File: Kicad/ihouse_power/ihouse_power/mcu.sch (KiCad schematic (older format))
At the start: 108 parts, among them J13 RJ33_Shielded, J20 Conn_02x05_Top_Bottom, J3 Conn_01x20, J4 Conn_01x20, M1 stm32f1_module, Q1 IRF7403, Q2 IRF7403, Q3 IRF7403, Q4 IRF7403, Q5 BC847, U10 MAX232, U11 L7805, U6 EL814, U7 EL814, U8 EL814, U9 24LC32

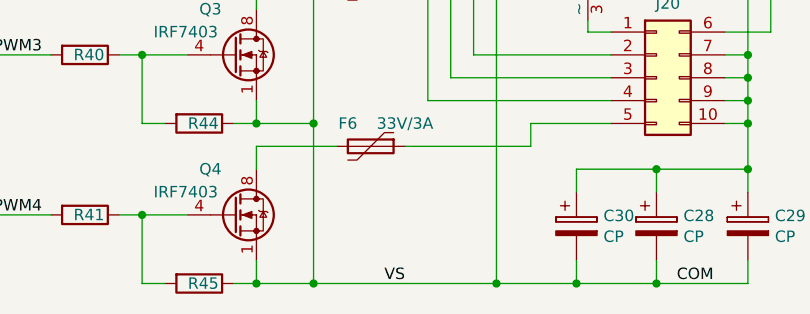
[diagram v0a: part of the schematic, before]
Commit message: schemos ir pcb paruosimas
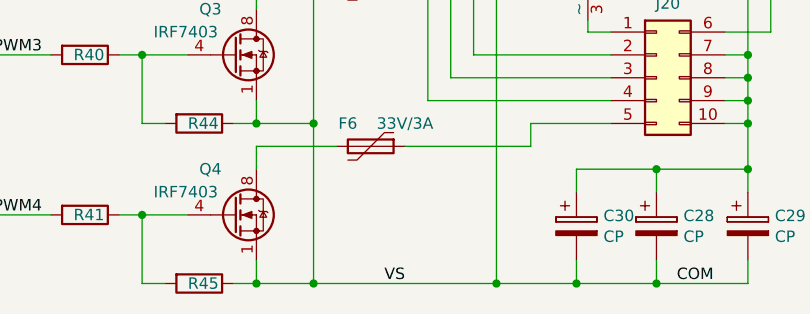
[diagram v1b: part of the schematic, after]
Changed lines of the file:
@@
 EESchema Schematic File Version 4
 LIBS:ihouse_power-cache
-EELAYER 26 0
+EELAYER 29 0
 EELAYER END
 $Descr A3 16535 11693
@@
 BUZMN
 Wire Wire Line
-	9300 10750 8900 10750
-Wire Wire Line
 	8900 8650 8900 9350
 Wire Wire Line
@@
 	9700 10750 10050 10750
 Wire Wire Line
-	9300 10750 9700 10750
+	8900 10750 9700 10750
 $EndSCHEMATC
